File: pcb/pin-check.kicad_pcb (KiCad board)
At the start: 2 copper layers, 114.3 x 44.2 mm, 56 parts, among them J1 AVR-ISP-6, P1 USB_C_Receptacle_USB2.0, SW1 SW_Push, SW2 SW_Push, SW3 SW_Push, SW4 SW_Push, SW5 SW_Push, SW6 SW_Push, SW7 Reset, SW8 Boot, U1 ATmega328P-PU, Y1 16MHz

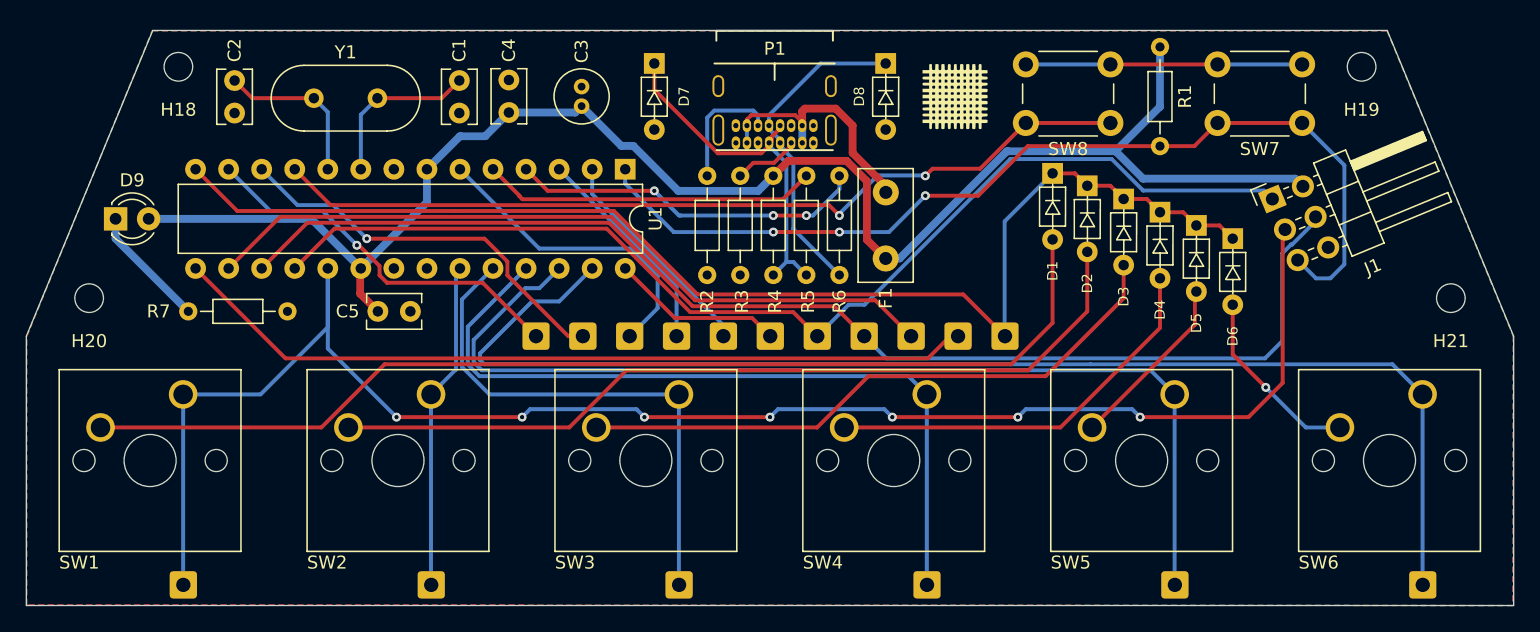
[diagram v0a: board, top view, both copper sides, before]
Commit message: smaller!
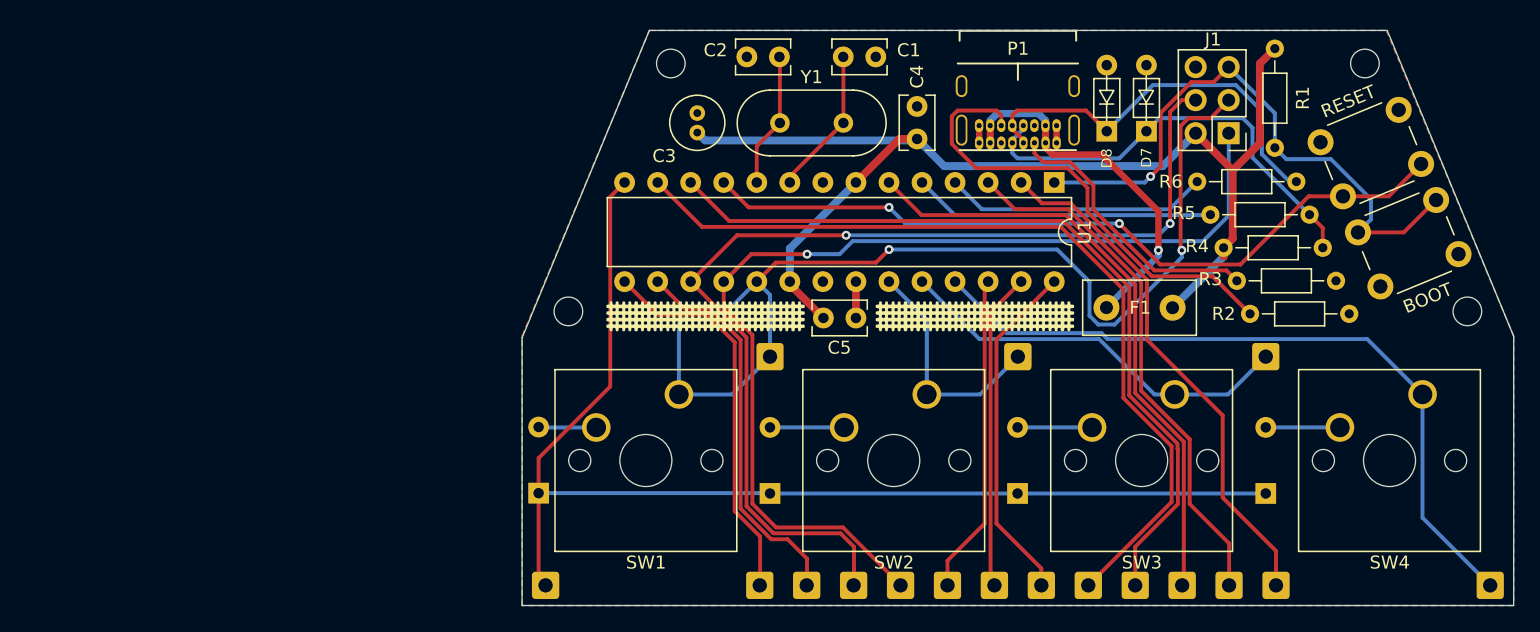
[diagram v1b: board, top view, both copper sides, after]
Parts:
- removed D5, D6: 1N4148, pin-check:D_DO-35_SOD27_P5.08mm_Horizontal
- removed D9: LED, LED_THT:LED_D3.0mm
- removed the G*** at (115.8, 38.6)
- removed R7: 1.5k, Resistor_THT:R_Axial_DIN0204_L3.6mm_D1.6mm_P7.62mm_Horizontal
- removed SW5, SW6: SW_Push, Button_Switch_Keyboard:SW_Cherry_MX_1.00u_PCB
- added G***: LOGO, pin-check:pin-check-pattern, F.Cu at (117.3, 55.5)
- added G***: LOGO, pin-check:pin-check-pattern, F.Cu at (96.6, 55.5)
- D1, D2, D3, D4: moved to B.Cu
- J1: footprint Connector_PinHeader_2.54mm:PinHeader_2x03_P2.54mm_Horizontal -> Connector_PinHeader_2.54mm:PinHeader_2x03_P2.54mm_Vertical
- moved H3 48.4 mm to (120.7, 58.6)
- moved H2 48.4 mm to (101.6, 58.6)
- moved H4 48.4 mm to (139.7, 58.6)
- moved D1 47.9 mm to (83.8, 70.4), turned to 90 degrees
- moved H5 43.3 mm to (156.9, 76.2)
- moved R2 43.0 mm to (138.5, 55.3), turned to 0 degrees
- moved H1 40.2 mm to (84.4, 76.2)
- moved C2 39.6 mm to (99.8, 35.6), turned to 0 degrees
- moved R3 39.0 mm to (137.5, 52.8), turned to 0 degrees
- moved D7 38.6 mm to (130.5, 42.5), turned to 90 degrees
- moved SW2 38.1 mm to (113.7, 61.5)
- moved SW1 38.1 mm to (94.6, 61.5)
- moved SW3 38.1 mm to (132.7, 61.5)
- moved SW4 38.1 mm to (151.8, 61.5)
- moved H18 37.8 mm to (94.0, 36.1)
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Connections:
- H10 pad 1: /B3 -> /D7
- H11 pad 1: /B4 -> /C5
- H12 pad 1: /C5 -> /C4
- H13 pad 1: /D0 -> /C3
- H14 pad 1: /D1 -> /B4
- H15 pad 1: /D4 -> /B3
- H16 pad 1: /D6 -> /B2
- H17 pad 1: /D7 -> /B1
- H6 pad 1: /Col4 -> /D0
- H7 pad 1: /Col5 -> /D1
- H8 pad 1: /B1 -> /D4
- H9 pad 1: /B2 -> /D6
- U1 pad 26: /Col4 -> /C3
- U1 pad 27: /Col5 -> /C4
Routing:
- net /Col5: track 100.1 -> 0.00 mm
- net /Col4: track 80.1 -> 0.00 mm
- net Net-(D1-Pad2): track 82.9 -> 4.44 mm
- net Net-(D2-Pad2): track 65.1 -> 5.70 mm
- net /Col0: track 128.6 -> 81.5 mm, vias 7 -> 2
- net Net-(D3-Pad2): track 47.2 -> 5.73 mm
- net /D7: track 29.4 -> 66.1 mm, vias 1 -> 0
- net +5V: track 124.2 -> 88.1 mm
- net /B1: track 62.1 -> 29.9 mm
- net /D6: track 30.6 -> 62.9 mm, vias 1 -> 0
- net /Reset: track 75.7 -> 46.5 mm, vias 3 -> 1
- net /B2: track 58.4 -> 29.9 mm
- net Net-(P1-PadB5): track 9.89 -> 36.5 mm
- net Net-(D4-Pad2): track 31.3 -> 5.70 mm
- net /C3: track 0.00 -> 24.6 mm
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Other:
- board size 114.3 x 44.2 mm -> 76.2 x 44.2 mm
- board text added: "BOOT"
- board text added: "RESET"
- board text added: "pin-check v0.1.0 by brian"
- board text removed: "pin-check v0.0.2 by brian"
